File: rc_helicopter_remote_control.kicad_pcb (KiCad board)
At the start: 2 copper layers, 39 parts, among them J1 SWD, SW1 SW_SPST, U1 STM32L4P5RET6, U2 LTC3440EMS, U3 NRF24L01_Breakout, Y1 16MHz

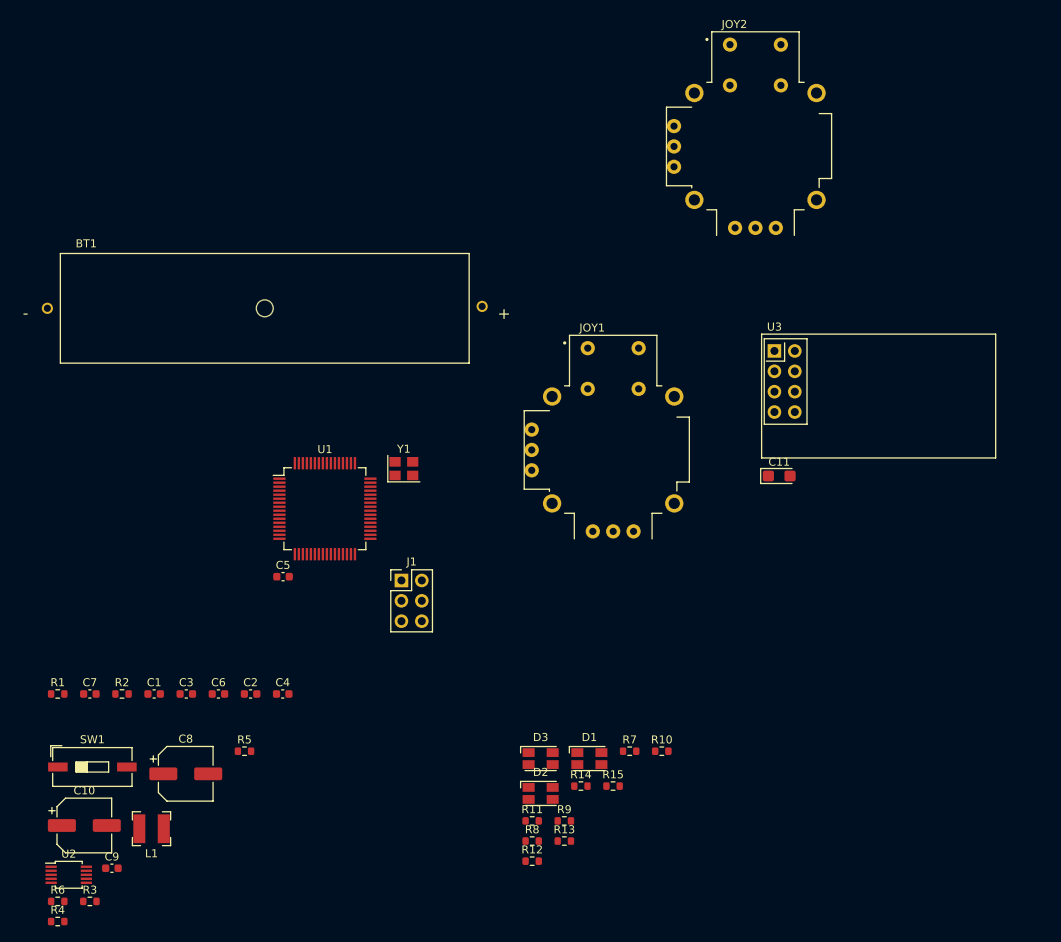
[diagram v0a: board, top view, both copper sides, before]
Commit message: Arrange footprints
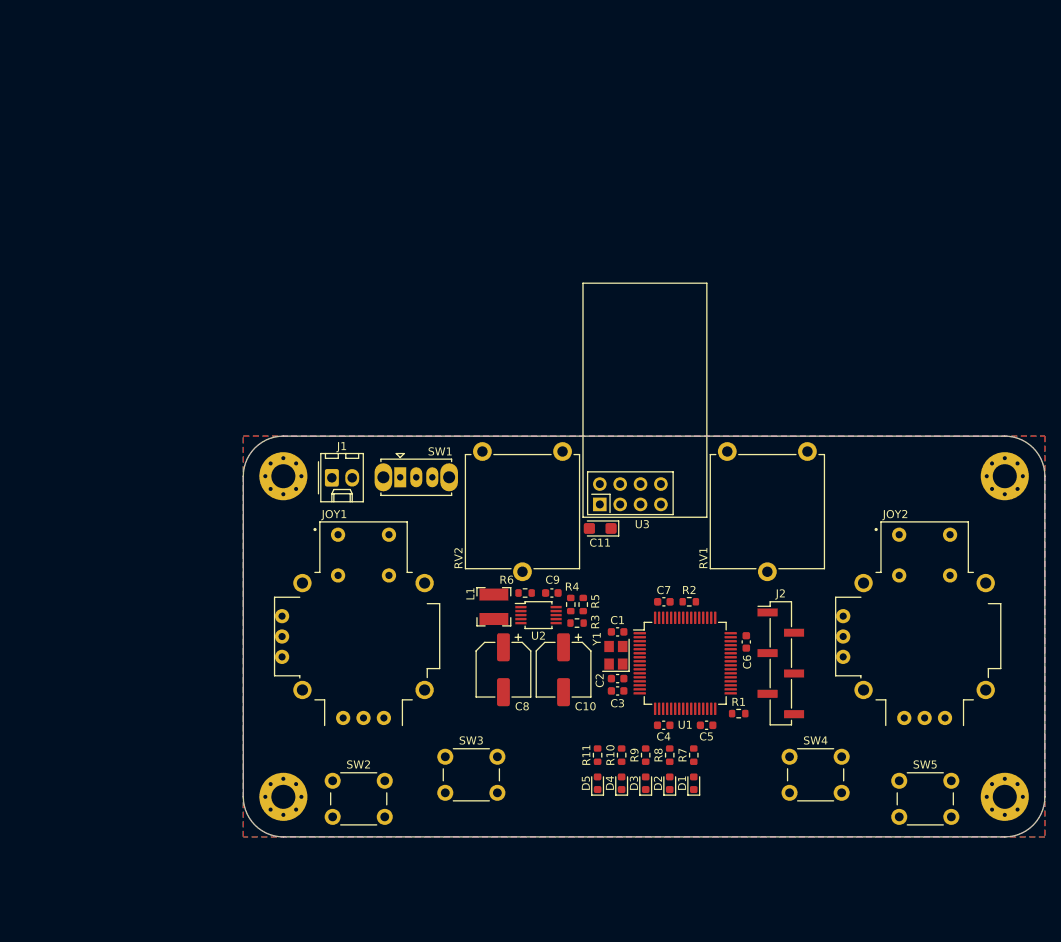
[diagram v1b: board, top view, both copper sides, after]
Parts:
- removed BT1: Li-Ion, Local_Library:BAT_BCAAAW
- removed R12, R13, R14, R15: 100Ω, Resistor_SMD:R_0603_1608Metric
- added D4: Blue, LED_SMD:LED_0603_1608Metric, F.Cu at (143.2, 118.3)
- added D5: Blue, LED_SMD:LED_0603_1608Metric, F.Cu at (140.2, 118.3)
- added J2: SWD, Connector_PinHeader_2.54mm:PinHeader_1x06_P2.54mm_Vertical_SMD_Pin1Left, F.Cu at (163.1, 103.3)
- added REF**: MountingHole_3mm_Pad_Via, MountingHole:MountingHole_3mm_Pad_Via, F.Cu at (191.0, 80.0)
- added REF**: MountingHole_3mm_Pad_Via, MountingHole:MountingHole_3mm_Pad_Via, F.Cu at (101.0, 80.0)
- added REF**: MountingHole_3mm_Pad_Via, MountingHole:MountingHole_3mm_Pad_Via, F.Cu at (101.0, 120.0)
- added REF**: MountingHole_3mm_Pad_Via, MountingHole:MountingHole_3mm_Pad_Via, F.Cu at (191.0, 120.0)
- added RV1: 100kΩ, Potentiometer_THT:Potentiometer_ACP_CA14V-15_Vertical, F.Cu at (156.4, 76.9)
- added RV2: 100kΩ, Potentiometer_THT:Potentiometer_ACP_CA14V-15_Vertical, F.Cu at (125.8, 76.9)
- added SW2: SW_Push, Button_Switch_THT:SW_PUSH_6mm_H13mm, F.Cu at (107.2, 118.0)
- added SW3: SW_Push, Button_Switch_THT:SW_PUSH_6mm_H13mm, F.Cu at (121.2, 115.0)
- added SW4: SW_Push, Button_Switch_THT:SW_PUSH_6mm_H13mm, F.Cu at (164.2, 115.0)
- added SW5: SW_Push, Button_Switch_THT:SW_PUSH_6mm_H13mm, F.Cu at (177.8, 118.0)
- D1, D2, D3: value LED_RGBK -> Blue; footprint LED_SMD:LED_Avago_PLCC4_3.2x2.8mm_CW -> LED_SMD:LED_0603_1608Metric
- J1: value SWD -> Battery Pack; footprint Connector_PinHeader_2.54mm:PinHeader_2x03_P2.54mm_Vertical -> Connector_Molex:Molex_KK-254_AE-6410-02A_1x02_P2.54mm_Vertical
- R10, R11: value 100Ω -> 140Ω
- R7, R8, R9: value 180Ω -> 140Ω
- SW1: footprint Button_Switch_SMD:SW_DIP_SPSTx01_Slide_9.78x4.72mm_W8.61mm_P2.54mm -> Button_Switch_THT:SW_Slide_1P2T_CK_OS102011MS2Q
- moved R1 85.0 mm to (157.8, 109.6)
- moved R4 75.2 mm to (136.9, 96.0), turned to 90 degrees
- moved C7 72.5 mm to (148.5, 95.7)
- moved R2 71.7 mm to (151.6, 95.7), turned to 180 degrees
- moved R3 70.0 mm to (137.6, 98.3)
- moved R6 69.9 mm to (131.2, 94.6), turned to 180 degrees
- moved U2 67.0 mm to (132.8, 97.3)
- moved C6 66.2 mm to (158.8, 100.7), turned to -90 degrees
- moved C9 64.7 mm to (134.5, 94.6)
- moved JOY2 64.7 mm to (181.0, 100.0)
- moved C10 62.9 mm to (136.0, 104.1), turned to -90 degrees
- moved C1 58.3 mm to (142.7, 99.4)
- moved C5 56.0 mm to (153.8, 111.1), turned to 180 degrees
- moved C3 53.8 mm to (142.7, 106.8)
- moved SW1 52.7 mm to (115.6, 80.1)
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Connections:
- C8 pad 1: GND -> +3.3V
- C8 pad 2: +3.3V -> GND
- D1 pad 1: Net-(D1-Pad1) -> GND
- D2 pad 1: Net-(D2-Pad1) -> GND
- D3 pad 1: Net-(D3-Pad1) -> GND
- J1 pad 1: +3.3V -> +BATT
- J1 pad 2: /SWCLK -> GND
- JOY2 pad 2: /JOY1_Y -> /JOY2_Y
- JOY2 pad 5: /JOY1_X -> /JOY2_X
- JOY2 pad 7: /JOY1_S -> /JOY2_S
- R10 pad 1: Net-(D1-Pad2) -> /LED4
- R10 pad 2: /LED1_G -> Net-(D4-Pad2)
- R11 pad 1: Net-(D2-Pad2) -> /LED5
- R11 pad 2: /LED2_G -> Net-(D5-Pad2)
- R7 pad 1: Net-(D1-Pad1) -> /LED1
- R7 pad 2: /LED1_R -> Net-(D1-Pad2)
- R8 pad 1: Net-(D2-Pad1) -> /LED2
- R8 pad 2: /LED2_R -> Net-(D2-Pad2)
- R9 pad 1: Net-(D3-Pad1) -> /LED3
- R9 pad 2: /LED3_R -> Net-(D3-Pad2)
- SW1 pad 1: /Power/+BATT -> Net-(C10-Pad1)
- SW1 pad 2: Net-(C10-Pad1) -> +BATT
- U1 pad 29: /LED2_R -> unconnected-(U1-Pad29)
- U1 pad 30: /LED2_G -> /LED1
- U1 pad 33: /LED2_B -> /LED2
- U1 pad 34: /LED3_R -> /LED3
- U1 pad 35: /LED3_G -> /LED4
- U1 pad 36: /LED3_B -> /LED5
- U1 pad 45: unconnected-(U1-Pad45) -> /POT1
- U1 pad 50: unconnected-(U1-Pad50) -> /POT2
- U1 pad 58: unconnected-(U1-Pad58) -> /SW1
- U1 pad 59: /LED1_R -> /SW2
- U1 pad 61: /LED1_G -> /SW3
- U1 pad 62: /LED1_B -> /SW4
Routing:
- added copper zone on B.Cu, net +3.3V
- added copper zone on F.Cu, net GND
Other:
- board outline added: 100 x 50 mm
